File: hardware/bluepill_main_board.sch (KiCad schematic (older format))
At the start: 2 parts

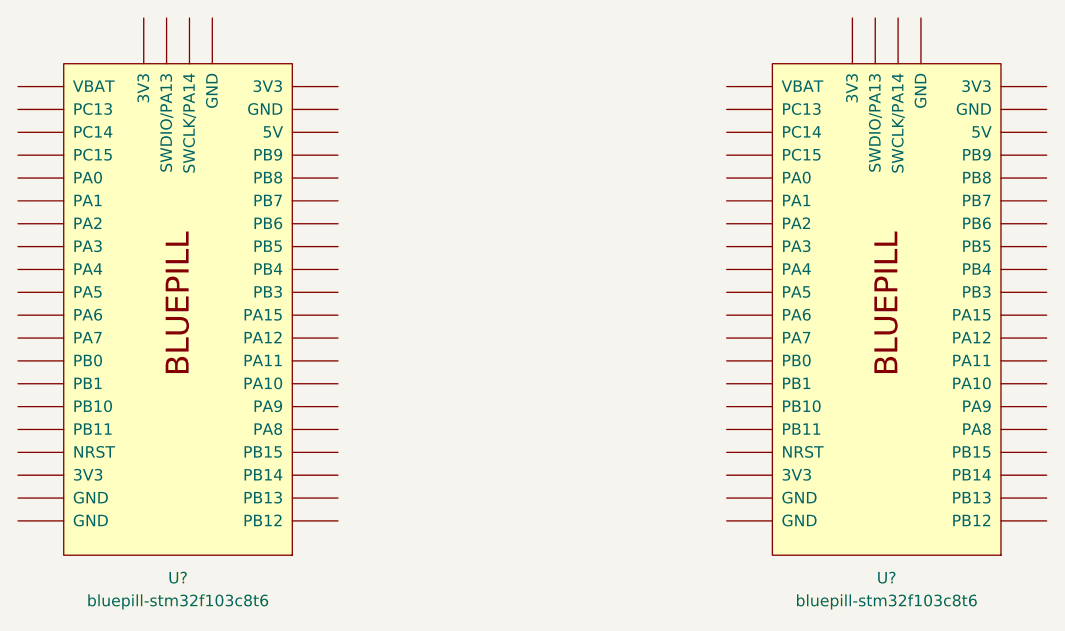
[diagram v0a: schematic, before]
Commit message: update,
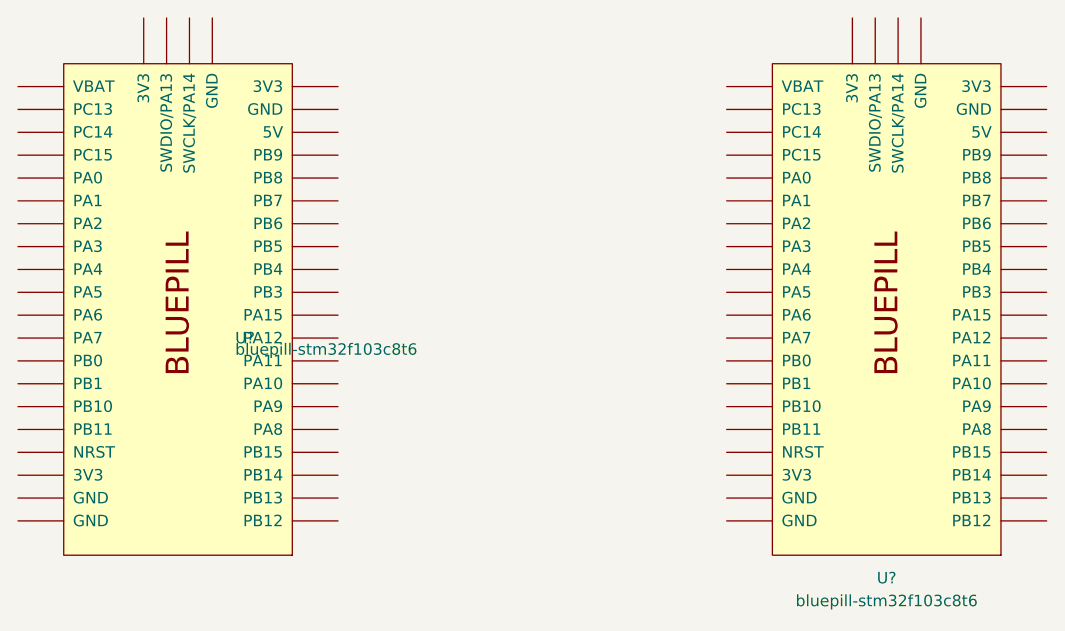
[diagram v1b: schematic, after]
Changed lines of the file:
@@
 $Descr A4 11693 8268
 encoding utf-8
-Sheet 4 17
+Sheet 4 22
 Title ""
 Date ""
@@
 U 1 1 5CDAC3D4
 P 4700 3750
-F 0 "U?" H 4700 4750 50  0000 C CNN
-F 1 "bluepill-stm32f103c8t6" H 4700 4850 50  0000 C CNN
+F 0 "U?" H 4450 3700 50  0000 R CNN
+F 1 "bluepill-stm32f103c8t6" H 4450 3750 50  0000 R CNN
 F 2 "" H 4700 3850 50  0001 C CNN
 F 3 "" H 4700 3850 50  0001 C CNN

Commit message: update,
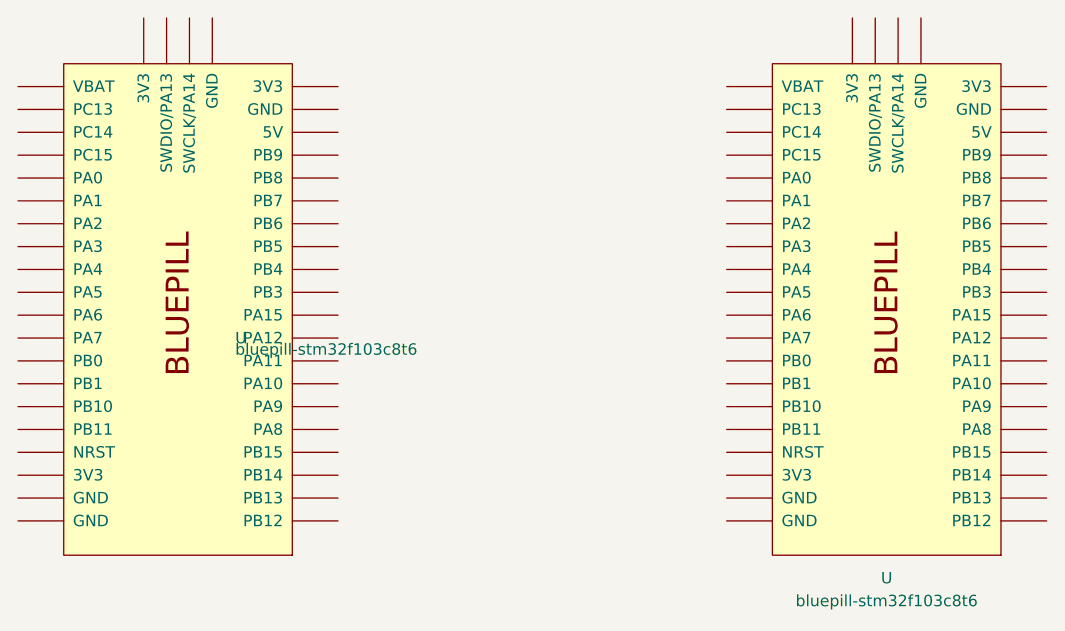
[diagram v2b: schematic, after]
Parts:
- U: renamed from U?; footprint (none) -> Package_DIP:DIP-40_W15.24mm_LongPads
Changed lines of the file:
@@
 $Descr A4 11693 8268
 encoding utf-8
-Sheet 4 22
+Sheet 4 23
 Title ""
 Date ""
@@
 $EndDescr
 $Comp
-L taobao-board:bluepill-stm32f103c8t6 U?
+L taobao-board:bluepill-stm32f103c8t6 U
 U 1 1 5CDAC3D4
 P 4700 3750
-F 0 "U?" H 4450 3700 50  0000 R CNN
+F 0 "U" H 4450 3700 50  0000 R CNN
 F 1 "bluepill-stm32f103c8t6" H 4450 3750 50  0000 R CNN
-F 2 "" H 4700 3850 50  0001 C CNN
+F 2 "Package_DIP:DIP-40_W15.24mm_LongPads" H 4700 3850 50  0001 C CNN
 F 3 "" H 4700 3850 50  0001 C CNN
 	1    4700 3750
@@
 $EndComp
 $Comp
-L taobao-board:bluepill-stm32f103c8t6 U?
+L taobao-board:bluepill-stm32f103c8t6 U
 U 1 1 5CDAE580
 P 7800 3750
-F 0 "U?" H 7800 4750 50  0000 C CNN
+F 0 "U" H 7800 4750 50  0000 C CNN
 F 1 "bluepill-stm32f103c8t6" H 7800 4850 50  0000 C CNN
-F 2 "" H 7800 3850 50  0001 C CNN
+F 2 "Package_DIP:DIP-40_W15.24mm_LongPads" H 7800 3850 50  0001 C CNN
 F 3 "" H 7800 3850 50  0001 C CNN
 	1    7800 3750
